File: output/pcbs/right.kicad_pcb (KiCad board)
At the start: 2 copper layers, 133.1 x 93.4 mm, 48 parts

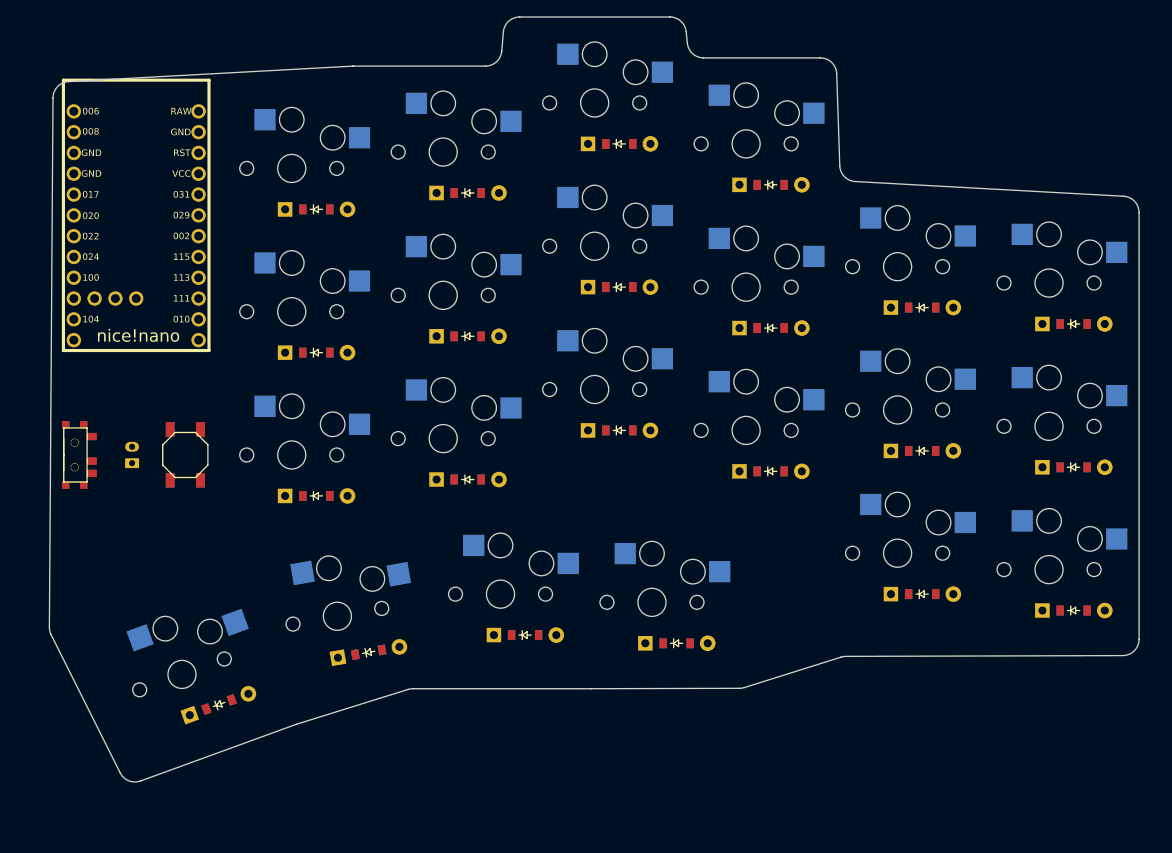
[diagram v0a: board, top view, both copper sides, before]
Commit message: More work on V2
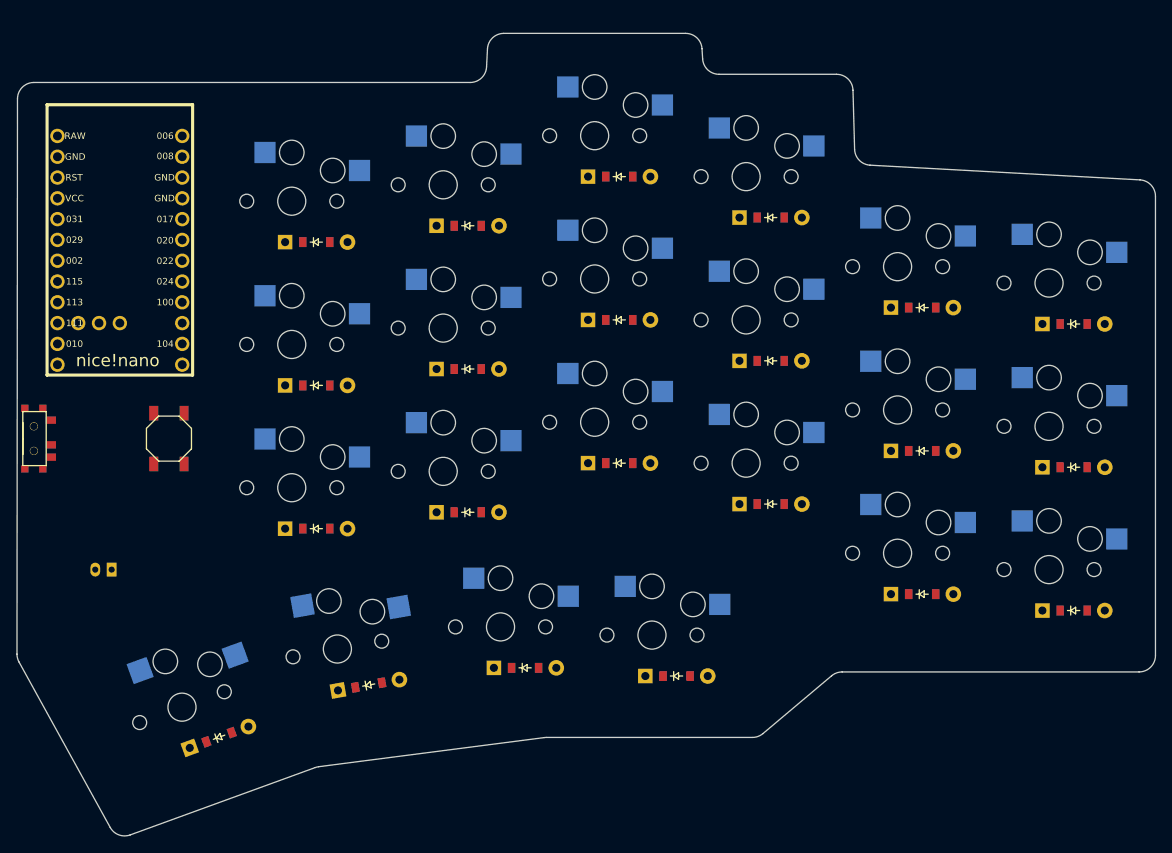
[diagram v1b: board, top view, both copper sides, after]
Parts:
- moved JST1 14.4 mm to (269.5, 82.5), turned to -180 degrees
- moved T1 5.39 mm to (261.0, 66.5)
- moved D10 4.00 mm to (332.5, 69.5)
- moved D11 4.00 mm to (332.5, 52.0)
- moved D12 4.00 mm to (332.5, 34.5)
- moved D13 4.00 mm to (314.0, 75.5)
- moved D14 4.00 mm to (314.0, 58.0)
- moved D15 4.00 mm to (314.0, 40.5)
- moved D16 4.00 mm to (295.5, 77.5)
- moved D17 4.00 mm to (295.5, 60.0)
- moved D18 4.00 mm to (295.5, 42.5)
- moved D19 4.00 mm to (339.5, 95.5)
- moved D20 4.00 mm to (321.0, 94.5)
- moved D21 4.00 mm to (301.9, 96.6)
- moved D22 4.00 mm to (283.6, 103.0)
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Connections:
- S1 pad 1: P031 -> P104
- S10 pad 1: P115 -> P002
- S11 pad 1: P115 -> P002
- S12 pad 1: P115 -> P002
- S13 pad 1: P113 -> P029
- S14 pad 1: P113 -> P029
- S15 pad 1: P113 -> P029
- S16 pad 1: P104 -> P031
- S17 pad 1: P104 -> P031
- S18 pad 1: P104 -> P031
- S19 pad 1: P002 -> P115
- S2 pad 1: P031 -> P104
- S20 pad 1: P115 -> P002
- S21 pad 1: P113 -> P029
- S22 pad 1: P104 -> P031
- S3 pad 1: P031 -> P104
- S4 pad 1: P029 -> P113
- S5 pad 1: P029 -> P113
- S6 pad 1: P029 -> P113
- S7 pad 1: P002 -> P115
- S8 pad 1: P002 -> P115
- S9 pad 1: P002 -> P115
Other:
- board size 133.1 x 93.4 mm -> 139.1 x 98 mm
